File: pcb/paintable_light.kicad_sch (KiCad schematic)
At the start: 29 parts, among them J1 USB_C_Receptacle_PowerOnly_6P, J2 Conn_01x01, J3 Conn_01x01, J4 Conn_01x01, U1 WS2811, U2 WS2811, U3 WS2811, U4 CH32V003JxMx

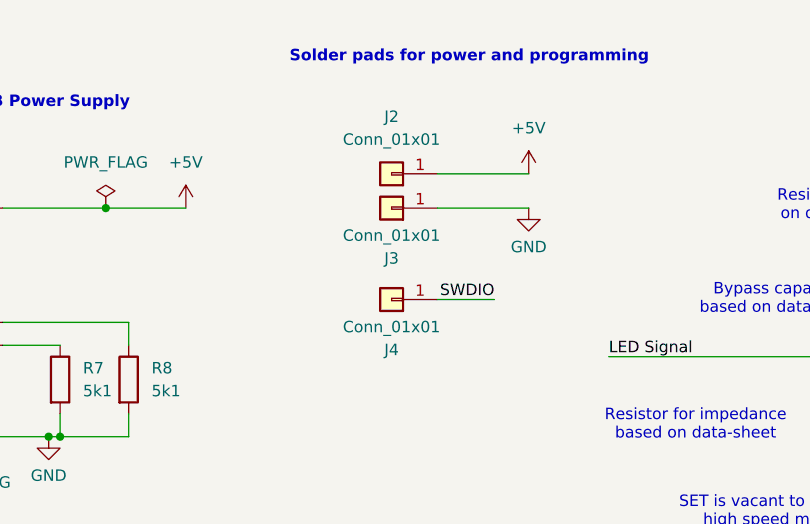
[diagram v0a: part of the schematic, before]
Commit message: v4
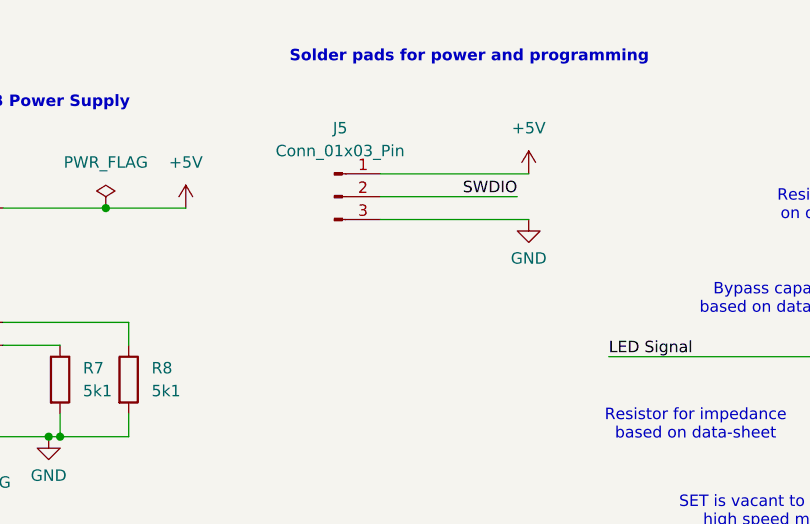
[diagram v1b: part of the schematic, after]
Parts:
- removed J2, J3, J4: Conn_01x01, TestPoint:TestPoint_Pad_2.5x2.5mm, symbol Connector_Generic:Conn_01x01
- added J5: Conn_01x03_Pin, front_leds:pin_header_flat_C41417360, symbol Connector:Conn_01x03_Pin
- J1: footprint front_leds:vertical_usb_c -> front_leds:usb_c_vertical_C5187465
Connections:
- net +5V: now also J5.1 (Pin_1)
- net GND: now also J5.3 (Pin_3)
- net SWDIO: now also J5.2 (Pin_2)
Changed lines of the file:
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@@
 	(wire
 		(pts
-			(xy 92.71 48.26) (xy 99.06 48.26)
-		)
-		(stroke
-			(width 0)
-			(type default)
-		)
-	)
-	(wire
-		(pts
 			(xy 50.8 63.5) (xy 49.53 63.5)
 		)
@@
 	(wire
 		(pts
-			(xy 92.71 34.29) (xy 102.87 34.29)
-		)
-		(stroke
-			(width 0)
-			(type default)
-		)
-	)
-	(wire
-		(pts
 			(xy 161.29 156.21) (xy 175.26 156.21)
 		)
@@
 	(wire
 		(pts
+			(xy 86.36 36.83) (xy 101.6 36.83)
+		)
+		(stroke
+			(width 0)
+			(type default)
+		)
+	)
+	(wire
+		(pts
 			(xy 182.88 161.29) (xy 191.77 161.29)
 		)
@@
 	(wire
 		(pts
+			(xy 86.36 34.29) (xy 102.87 34.29)
+		)
+		(stroke
+			(width 0)
+			(type default)
+		)
+	)
+	(wire
+		(pts
 			(xy 58.42 63.5) (xy 50.8 63.5)
 		)
@@
 	(wire
 		(pts
-			(xy 92.71 38.1) (xy 102.87 38.1)
+			(xy 44.45 38.1) (xy 55.88 38.1)
 		)
 		(stroke
@@
 	(wire
 		(pts
-			(xy 44.45 38.1) (xy 55.88 38.1)
+			(xy 58.42 50.8) (xy 58.42 53.34)
 		)
 		(stroke
@@
 	(wire
 		(pts
-			(xy 58.42 50.8) (xy 58.42 53.34)
+			(xy 161.29 64.77) (xy 175.26 64.77)
 		)
 		(stroke
@@
 	(wire
 		(pts
-			(xy 161.29 64.77) (xy 175.26 64.77)
+			(xy 151.13 41.91) (xy 151.13 48.26)
 		)
 		(stroke
@@
 	(wire
 		(pts
-			(xy 151.13 41.91) (xy 151.13 48.26)
+			(xy 182.88 69.85) (xy 191.77 69.85)
 		)
 		(stroke
@@
 	(wire
 		(pts
-			(xy 182.88 69.85) (xy 191.77 69.85)
+			(xy 86.36 39.37) (xy 102.87 39.37)
 		)
 		(stroke
@@
 	)
 	(label "SWDIO"
-		(at 99.06 48.26 180)
+		(at 101.6 36.83 180)
 		(effects
 			(font
@@
 	)
 	(symbol
-		(lib_id "Connector_Generic:Conn_01x01")
-		(at 87.63 48.26 180)
-		(unit 1)
-		(body_style 1)
-		(exclude_from_sim no)
-		(in_bom no)
-		(on_board yes)
-		(in_pos_files yes)
-		(dnp no)
-		(property "Reference" "J4"
-			(at 87.63 53.848 0)
-			(show_name no)
-			(do_not_autoplace no)
-			(effects
-				(font
-					(size 1.27 1.27)
-				)
-			)
-		)
-		(property "Value" "Conn_01x01"
-			(at 87.63 51.308 0)
-			(show_name no)
-			(do_not_autoplace no)
-			(effects
-				(font
-					(size 1.27 1.27)
-				)
-			)
-		)
-		(property "Footprint" "TestPoint:TestPoint_Pad_2.5x2.5mm"
-			(at 87.63 48.26 0)
-			(hide yes)
-			(show_name no)
-			(do_not_autoplace no)
-			(effects
-				(font
-					(size 1.27 1.27)
-				)
-			)
-		)
-		(property "Datasheet" ""
-			(at 87.63 48.26 0)
-			(hide yes)
-			(show_name no)
-			(do_not_autoplace no)
-			(effects
-				(font
-					(size 1.27 1.27)
-				)
-			)
-		)
-		(property "Description" "Generic connector, single row, 01x01, script generated (kicad-library-utils/schlib/autogen/connector/)"
-			(at 87.63 48.26 0)
-			(hide yes)
-			(show_name no)
-			(do_not_autoplace no)
-			(effects
-				(font
-					(size 1.27 1.27)
-				)
-			)
-		)
-		(pin "1"
-		)
-		(instances
-			(project "paintable_light"
-				(path "/457c06ef-ae7c-4900-b3d7-3510fa92c411"
-					(reference "J4")
-					(unit 1)
-				)
-			)
-		)
-	)
-	(symbol
 		(lib_id "power:GND")
 		(at 143.51 143.51 0)
@@
 	)
 	(symbol
-		(lib_id "Connector_Generic:Conn_01x01")
-		(at 87.63 38.1 180)
-		(unit 1)
-		(body_style 1)
-		(exclude_from_sim no)
-		(in_bom no)
-		(on_board yes)
-		(in_pos_files yes)
-		(dnp no)
-		(property "Reference" "J3"
-			(at 87.63 43.688 0)
-			(show_name no)
-			(do_not_autoplace no)
-			(effects
-				(font
-					(size 1.27 1.27)
-				)
-			)
-		)
-		(property "Value" "Conn_01x01"
-			(at 87.63 41.148 0)
-			(show_name no)
-			(do_not_autoplace no)
-			(effects
-				(font
-					(size 1.27 1.27)
-				)
-			)
-		)
-		(property "Footprint" "TestPoint:TestPoint_Pad_2.5x2.5mm"
-			(at 87.63 38.1 0)
-			(hide yes)
-			(show_name no)
-			(do_not_autoplace no)
-			(effects
-				(font
-					(size 1.27 1.27)
-				)
-			)
-		)
-		(property "Datasheet" ""
-			(at 87.63 38.1 0)
-			(hide yes)
-			(show_name no)
-			(do_not_autoplace no)
-			(effects
-				(font
-					(size 1.27 1.27)
-				)
-			)
-		)
-		(property "Description" "Generic connector, single row, 01x01, script generated (kicad-library-utils/schlib/autogen/connector/)"
-			(at 87.63 38.1 0)
-			(hide yes)
-			(show_name no)
-			(do_not_autoplace no)
-			(effects
-				(font
-					(size 1.27 1.27)
-				)
-			)
-		)
-		(pin "1"
-		)
-		(instances
-			(project "paintable_light"
-				(path "/457c06ef-ae7c-4900-b3d7-3510fa92c411"
-					(reference "J3")
-					(unit 1)
-				)
-			)
-		)
-	)
-	(symbol
 		(lib_id "power:+5V")
 		(at 67.31 101.6 0)
@@
 	)
 	(symbol
+		(lib_id "Connector:Conn_01x03_Pin")
+		(at 81.28 36.83 0)
+		(unit 1)
+		(body_style 1)
+		(exclude_from_sim no)
+		(in_bom yes)
+		(on_board yes)
+		(in_pos_files yes)
+		(dnp no)
+		(fields_autoplaced yes)
+		(property "Reference" "J5"
+			(at 81.915 29.21 0)
+			(show_name no)
+			(do_not_autoplace no)
+			(effects
+				(font
+					(size 1.27 1.27)
+				)
+			)
+		)
+		(property "Value" "Conn_01x03_Pin"
+			(at 81.915 31.75 0)
+			(show_name no)
+			(do_not_autoplace no)
+			(effects
+				(font
+					(size 1.27 1.27)
+				)
+			)
+		)
+		(property "Footprint" "front_leds:pin_header_flat_C41417360"
+			(at 81.28 36.83 0)
+			(hide yes)
+			(show_name no)
+			(do_not_autoplace no)
+			(effects
+				(font
+					(size 1.27 1.27)
+				)
+			)
+		)
+		(property "Datasheet" ""
+			(at 81.28 36.83 0)
+			(hide yes)
+			(show_name no)
+			(do_not_autoplace no)
+			(effects
+				(font
+					(size 1.27 1.27)
+				)
+			)
+		)
+		(property "Description" "Generic connector, single row, 01x03, script generated"
+			(at 81.28 36.83 0)
+			(hide yes)
+			(show_name no)
+			(do_not_autoplace no)
+			(effects
+				(font
+					(size 1.27 1.27)
+				)
+			)
+		)
+		(pin "2"
+		)
+		(pin "3"
+		)
+		(pin "1"
+		)
+		(instances
+			(project "paintable_light"
+				(path "/457c06ef-ae7c-4900-b3d7-3510fa92c411"
+					(reference "J5")
+					(unit 1)
+				)
+			)
+		)
+	)
+	(symbol
 		(lib_id "Device:C")
 		(at 147.32 97.79 90)
@@
 			)
 		)
-		(property "Footprint" "front_leds:vertical_usb_c"
+		(property "Footprint" "front_leds:usb_c_vertical_C5187465"
 			(at 33.02 43.18 0)
 			(hide yes)
@@
 	(symbol
 		(lib_id "power:GND")
-		(at 102.87 38.1 0)
+		(at 102.87 39.37 0)
 		(unit 1)
 		(body_style 1)
@@
 		(dnp no)
 		(property "Reference" "#PWR018"
-			(at 102.87 44.45 0)
+			(at 102.87 45.72 0)
 			(hide yes)
 			(show_name no)
@@
 		)
 		(property "Value" "GND"
-			(at 102.87 42.418 0)
+			(at 102.87 43.688 0)
 			(show_name no)
 			(do_not_autoplace no)
@@
 		)
 		(property "Footprint" ""
-			(at 102.87 38.1 0)
+			(at 102.87 39.37 0)
 			(hide yes)
 			(show_name no)
@@
 		)
 		(property "Datasheet" ""
-			(at 102.87 38.1 0)
+			(at 102.87 39.37 0)
 			(hide yes)
 			(show_name no)
@@
 		)
 		(property "Description" "Power symbol creates a global label with name \"GND\" , ground"
-			(at 102.87 38.1 0)
+			(at 102.87 39.37 0)
 			(hide yes)
 			(show_name no)
@@
 					(unit 1)
 				)
-			)
-		)
-	)
-	(symbol
-		(lib_id "Connector_Generic:Conn_01x01")
-		(at 87.63 34.29 180)
-		(unit 1)
-		(body_style 1)
-		(exclude_from_sim no)
-		(in_bom no)
-		(on_board yes)
-		(in_pos_files yes)
-		(dnp no)
-		(fields_autoplaced yes)
-		(property "Reference" "J2"
-			(at 87.63 27.94 0)
-			(show_name no)
-			(do_not_autoplace no)
-			(effects
-				(font
-					(size 1.27 1.27)
-				)
-			)
-		)
-		(property "Value" "Conn_01x01"
-			(at 87.63 30.48 0)
-			(show_name no)
-			(do_not_autoplace no)
-			(effects
-				(font
-					(size 1.27 1.27)
-				)
-			)
-		)
-		(property "Footprint" "TestPoint:TestPoint_Pad_2.5x2.5mm"
-			(at 87.63 34.29 0)
-			(hide yes)
-			(show_name no)
-			(do_not_autoplace no)
-			(effects
-				(font
-					(size 1.27 1.27)
-				)
-			)
-		)
-		(property "Datasheet" ""
-			(at 87.63 34.29 0)
-			(hide yes)
-			(show_name no)
-			(do_not_autoplace no)
-			(effects
-				(font
-					(size 1.27 1.27)
-				)
-			)
-		)
-		(property "Description" "Generic connector, single row, 01x01, script generated (kicad-library-utils/schlib/autogen/connector/)"
-			(at 87.63 34.29 0)
-			(hide yes)
-			(show_name no)
-			(do_not_autoplace no)
-			(effects
-				(font
-					(size 1.27 1.27)
-				)
-			)
-		)
-		(pin "1"
-		)
-		(instances
-			(project "paintable_light"
-				(path "/457c06ef-ae7c-4900-b3d7-3510fa92c411"
-					(reference "J2")
-					(unit 1)
-				)
